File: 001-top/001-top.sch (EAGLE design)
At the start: 64 parts, among them J1 5267-5, U2 PCA9555PW,112

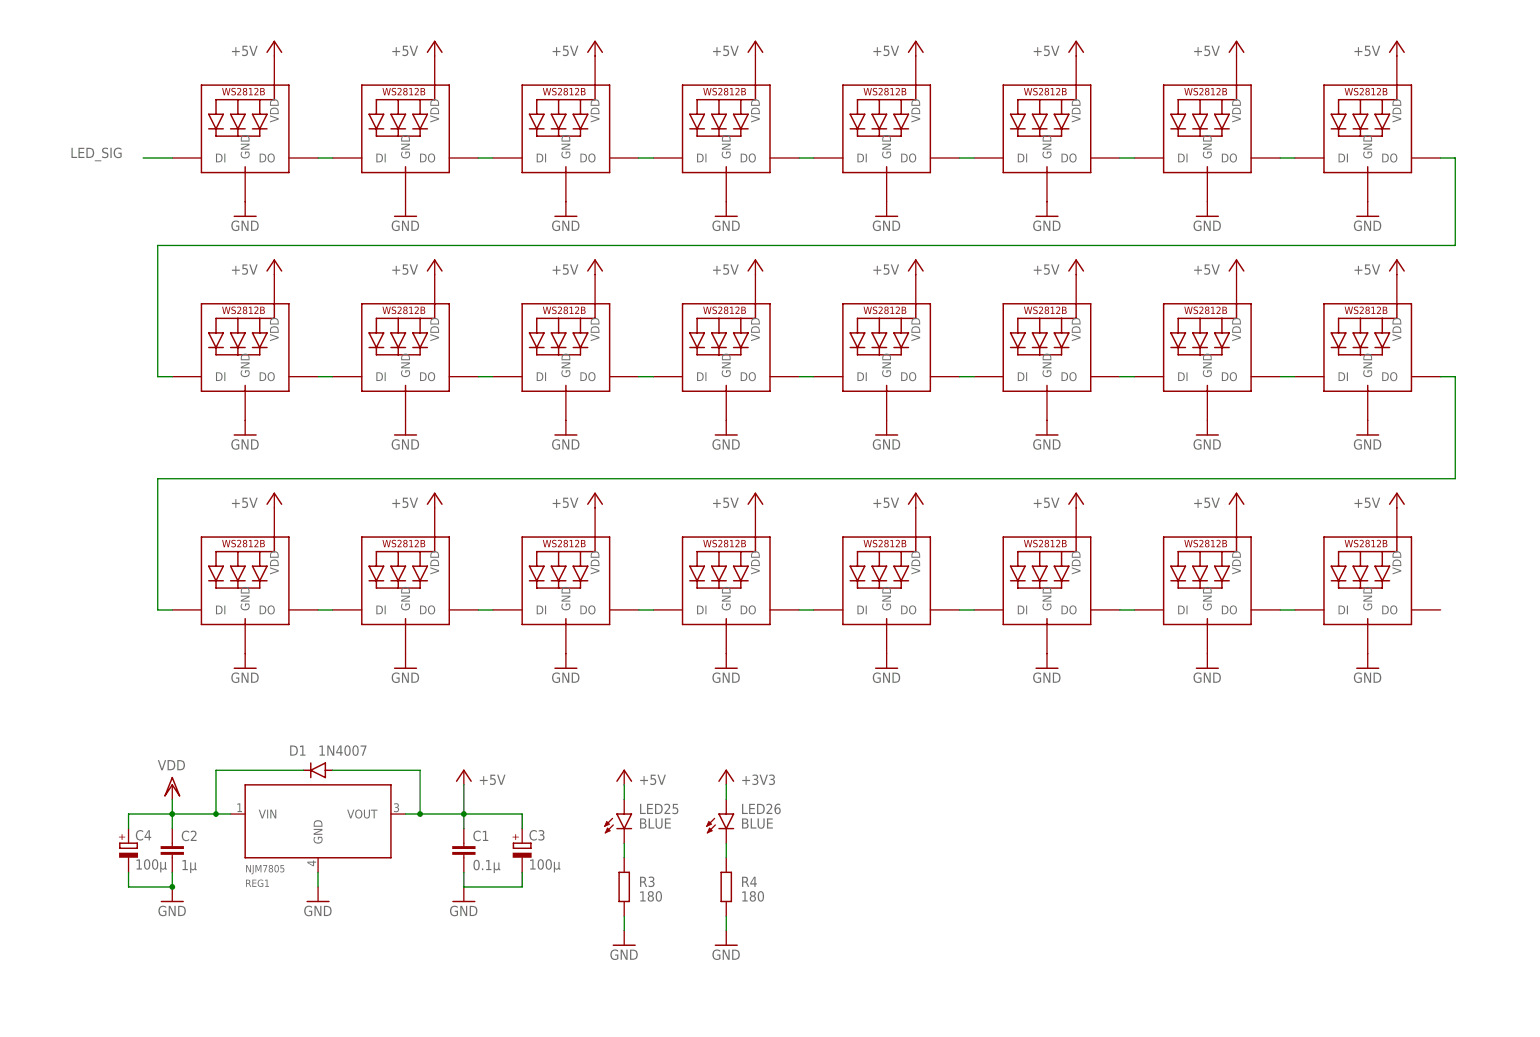
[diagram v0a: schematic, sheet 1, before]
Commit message: #WeLoveSTM32
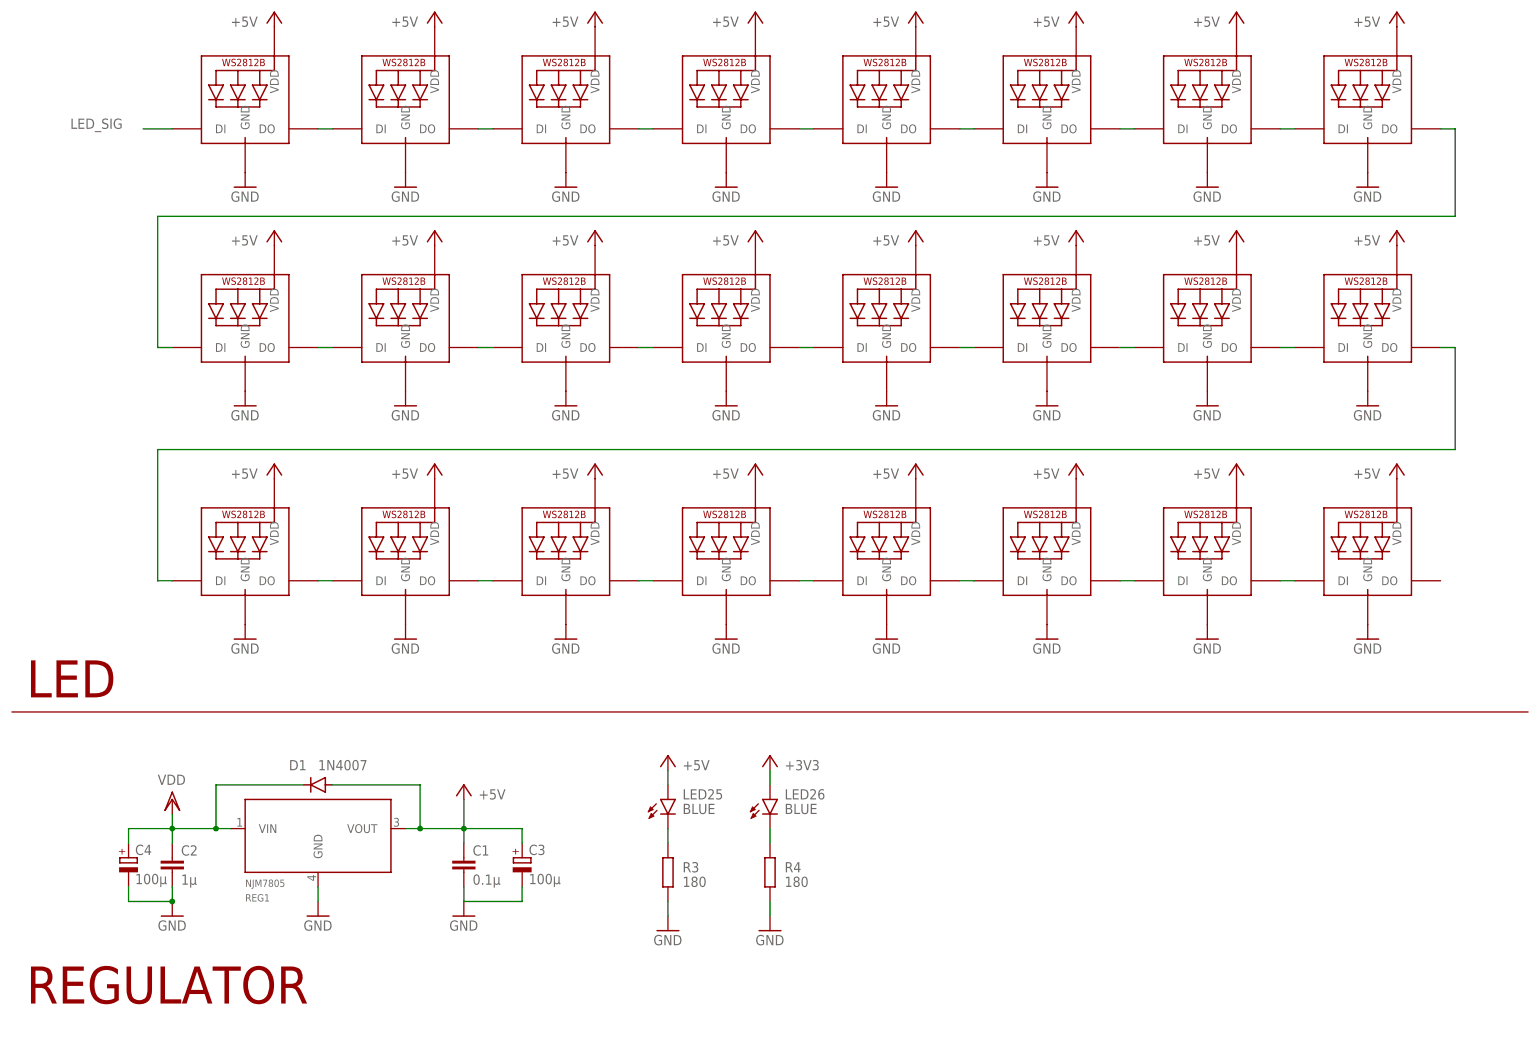
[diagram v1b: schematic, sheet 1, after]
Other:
- note added: "CONN"
- note added: "LED"
- note added: "PCA9555"
- note added: "PULL UP"
- note added: "REGULATOR"
- note added: "VL53L0X"
- note added: "XIAO"
- moved on the sheet: C1, C2, C3, C4, D1, J1, LED25, LED26, R1, R10, R11, R12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
